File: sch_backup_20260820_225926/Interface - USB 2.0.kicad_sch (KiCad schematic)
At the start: 20 parts, among them J10 TYPE-C 16PIN 2MD, J9 TYPE-C 16PIN 2MD

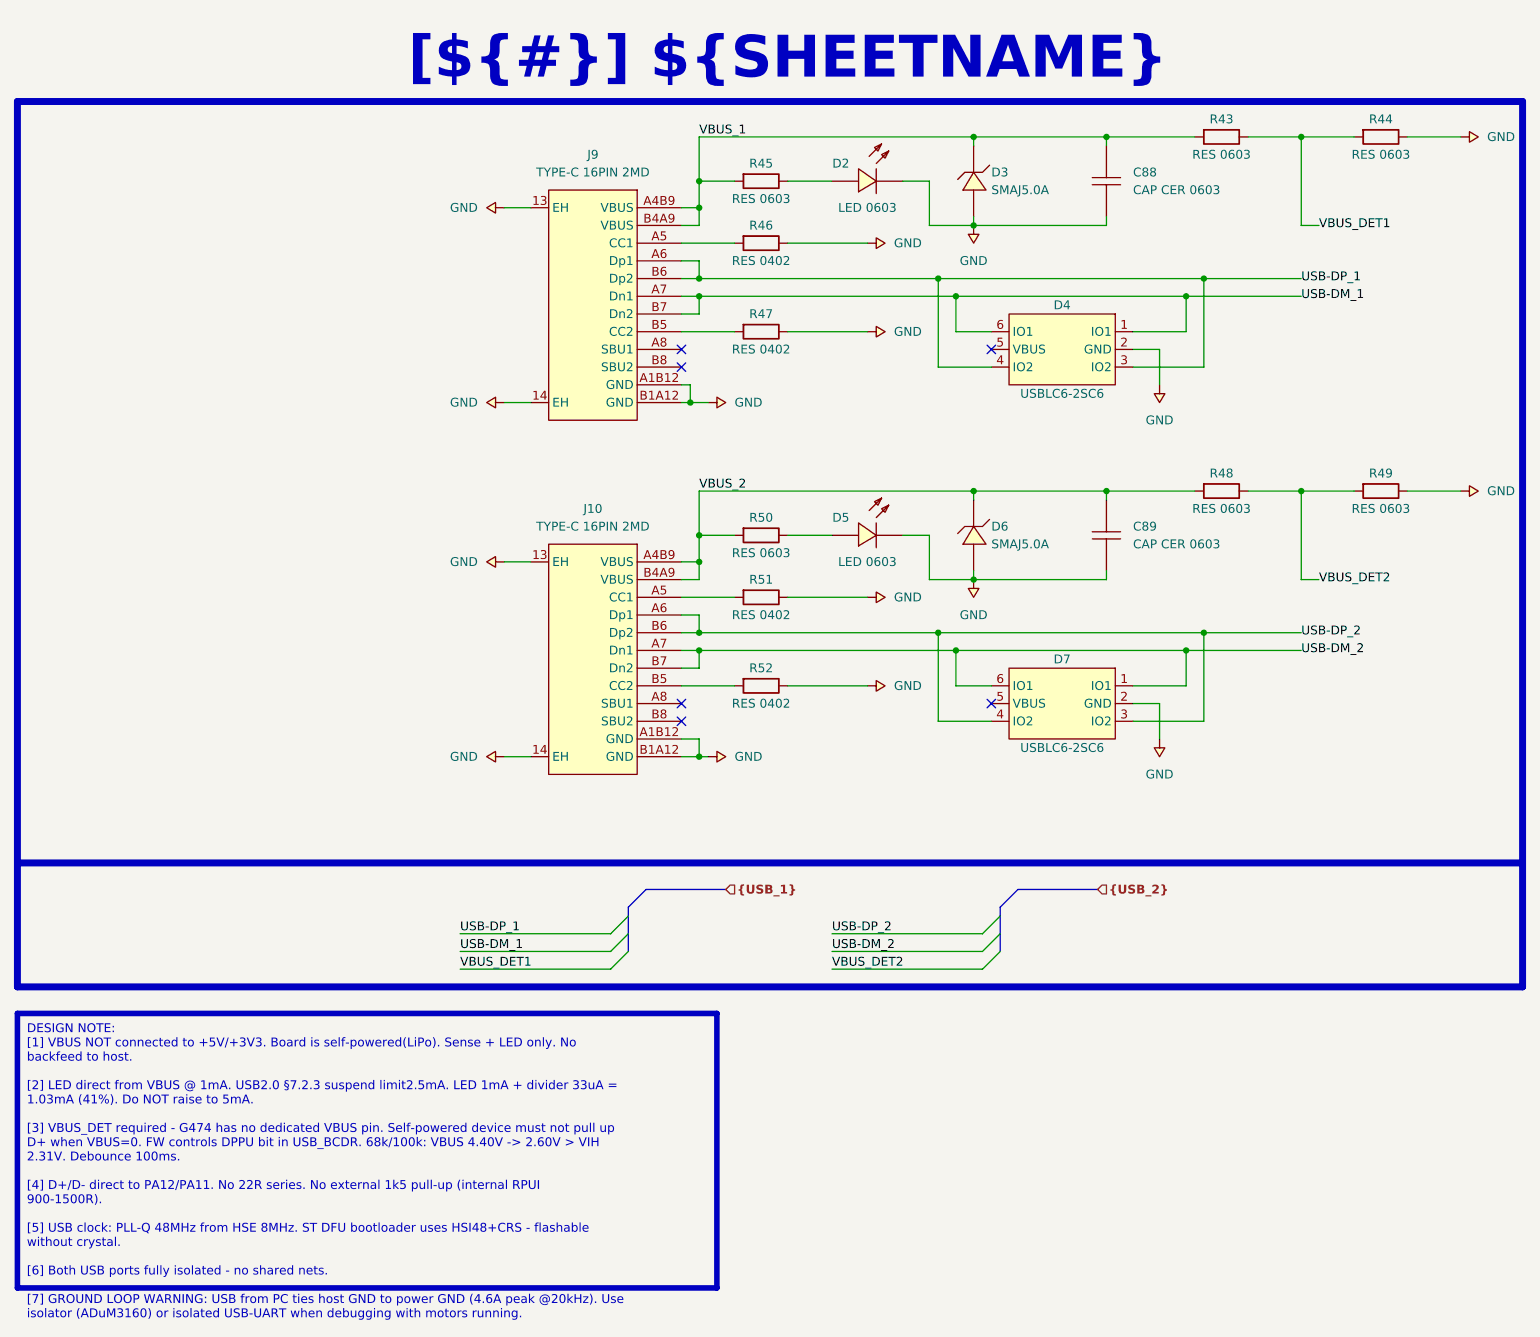
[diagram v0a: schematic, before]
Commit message: Update Schematic
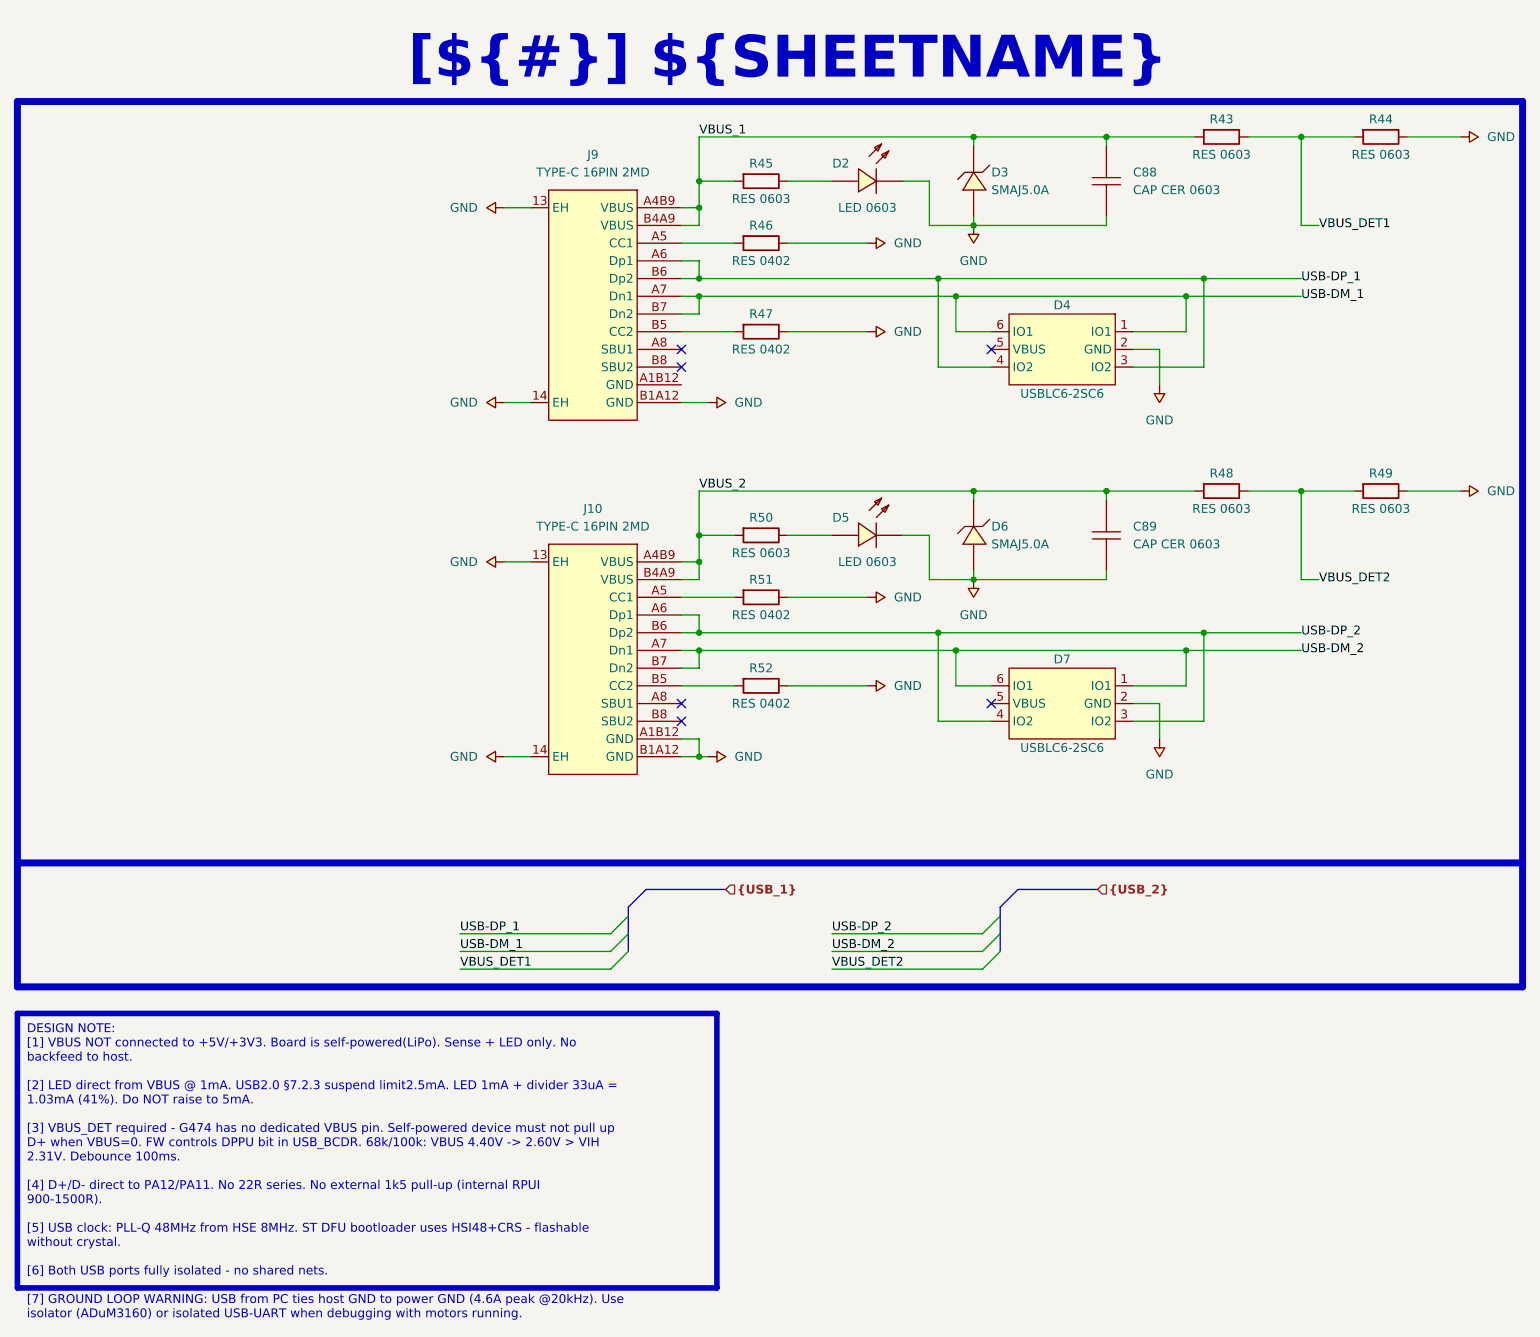
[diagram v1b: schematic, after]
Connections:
- net GND: no longer J9.A1B12 (GND)
